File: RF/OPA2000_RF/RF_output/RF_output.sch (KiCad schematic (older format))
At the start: 36 parts, among them J1 Conn_Coaxial, J2 VDD in, J3 GND, Q1 BLF188XR, T1 TLT, T2 TLT, T3 TLT

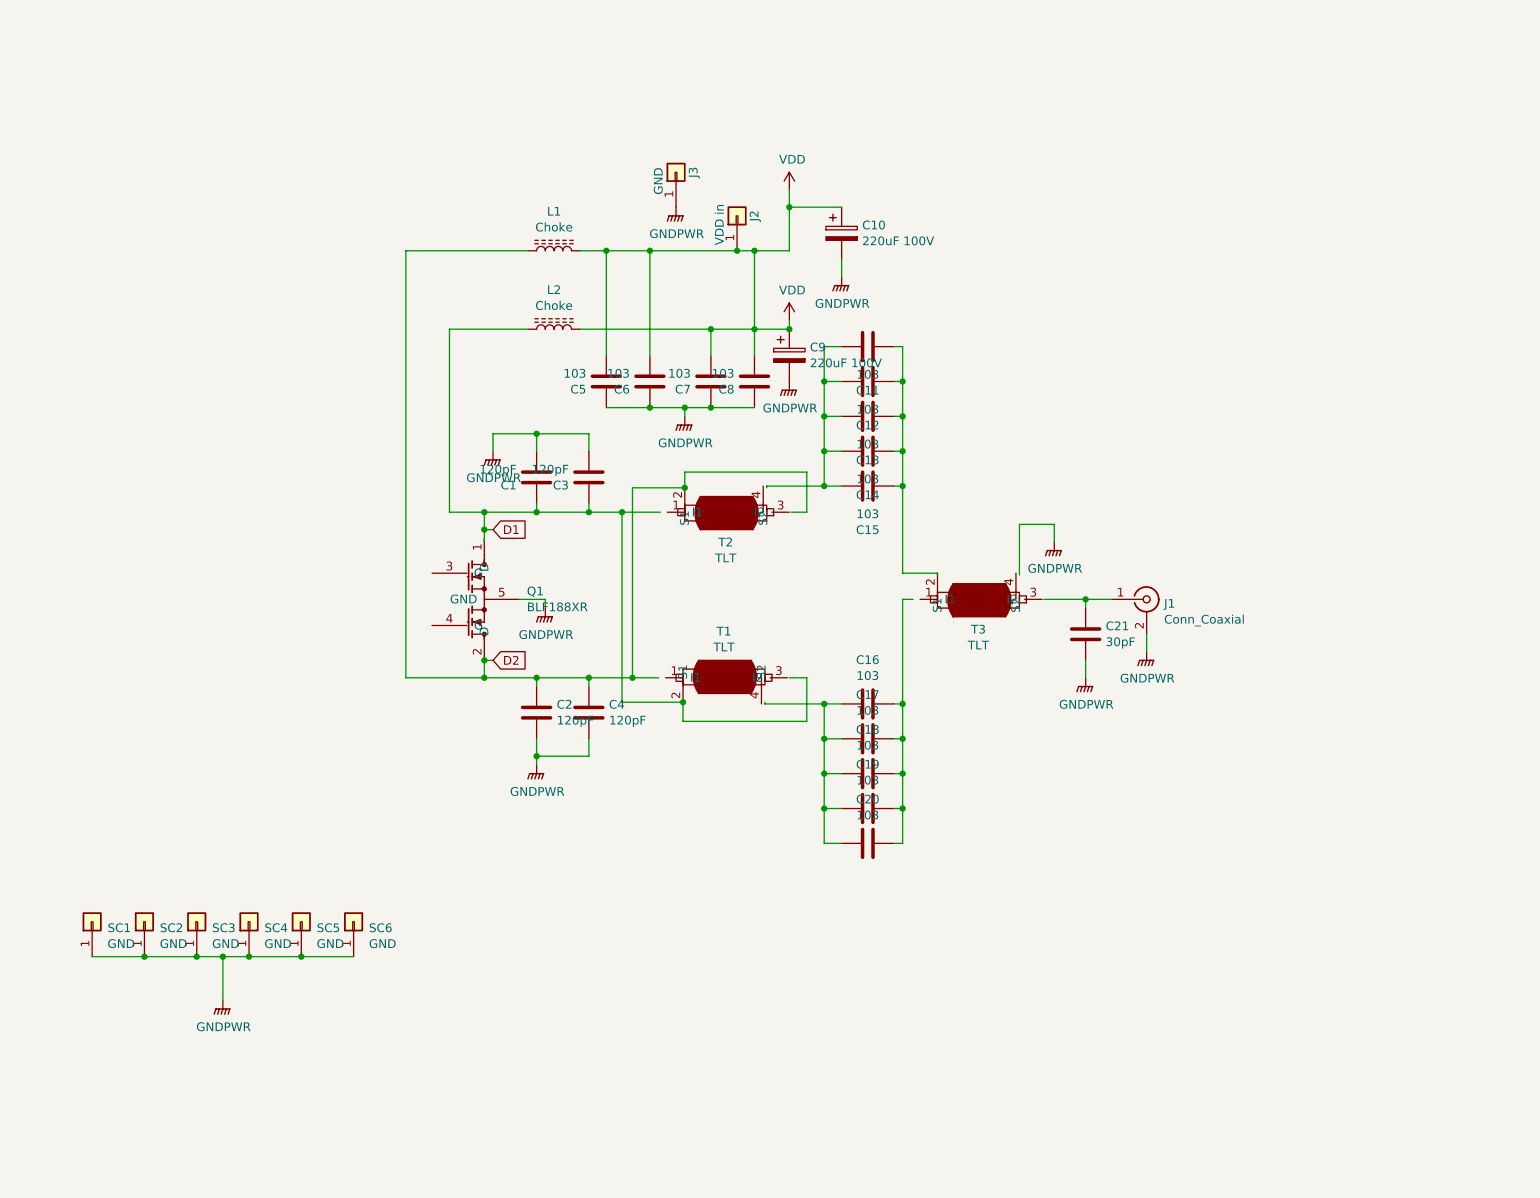
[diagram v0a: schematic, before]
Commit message: MCU2 sch done
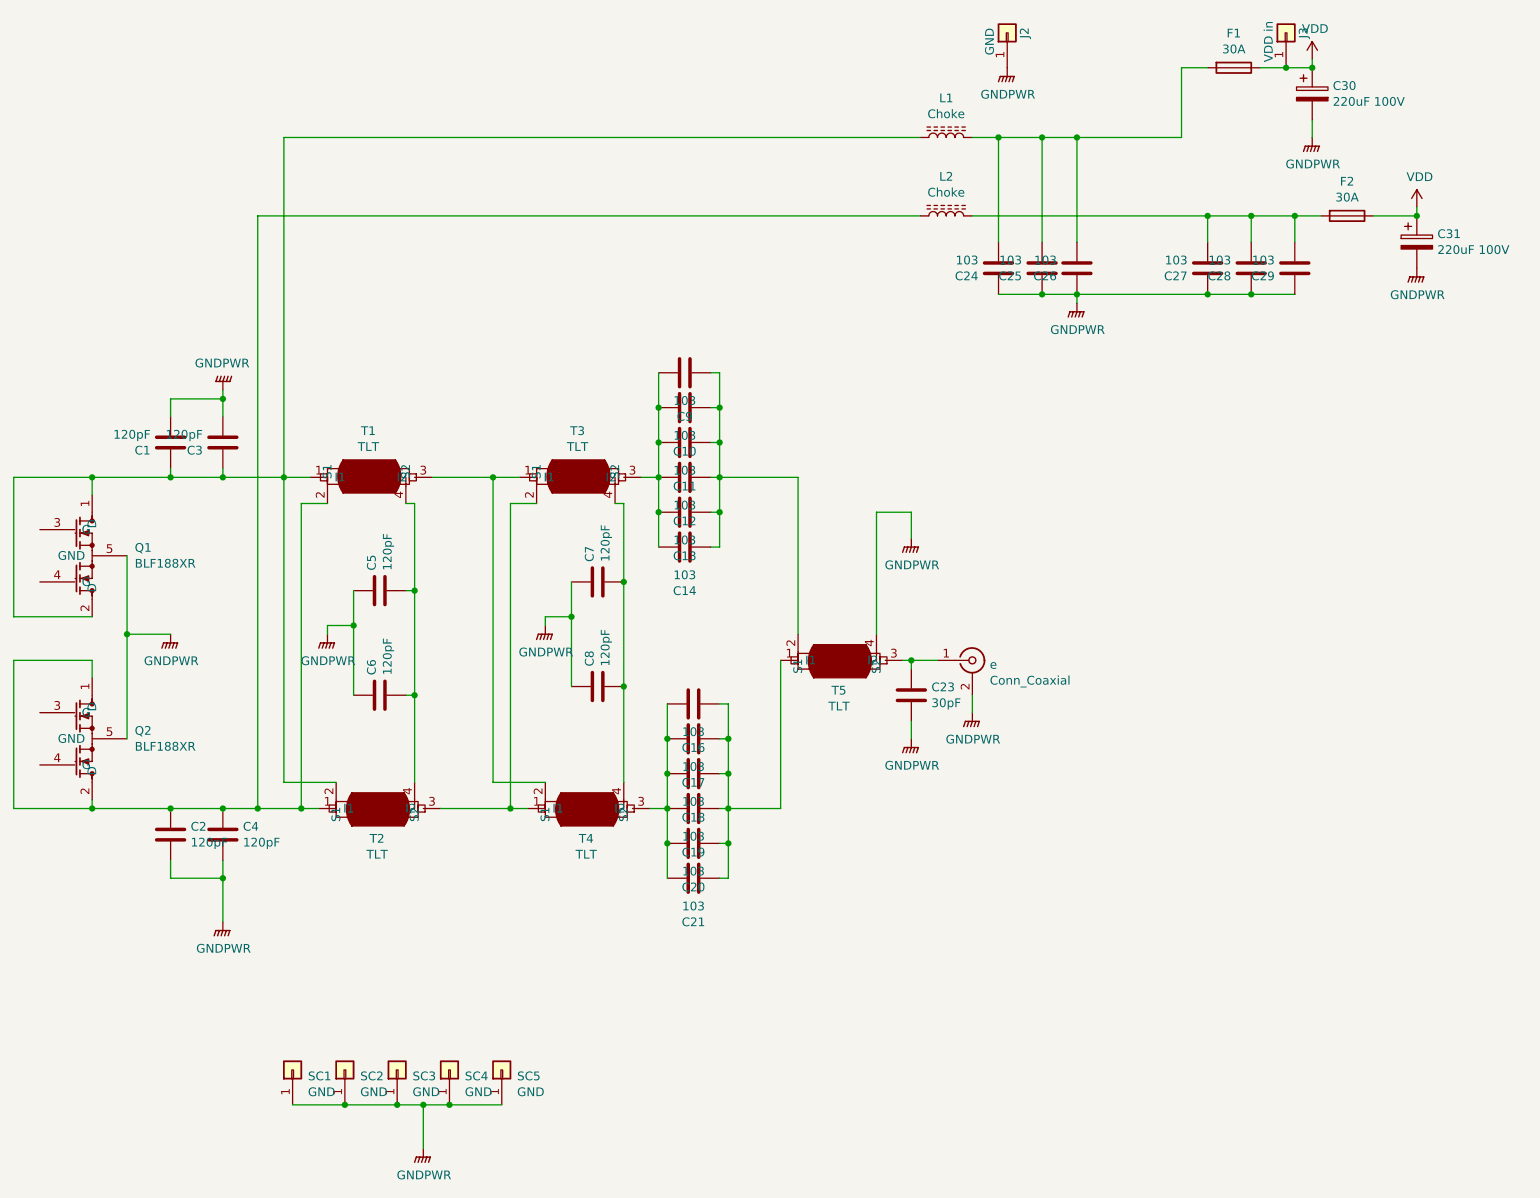
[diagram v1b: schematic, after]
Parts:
- removed C15: 103, Capacitors_SMD:C_1206_HandSoldering, symbol Device:C
- removed SC6: GND, MyPCBLib:M3_Screwhole, symbol Connector_Generic:Conn_01x01
- added C10, C21, C26, C29, C9: 103, Capacitor_SMD:C_1206_3216Metric_Pad1.33x1.80mm_HandSolder, symbol Device:C
- added C5, C6, C7, C8: 120pF, Capacitor_SMD:C_1210_3225Metric_Pad1.33x2.70mm_HandSolder, symbol Device:C
- added F1, F2: 30A, MyPCBLib:Fuseholder_Littelfuse_Nano2_456, symbol Device:Fuse
- added Q2: BLF188XR, MyPCBLib:BLF188XR, symbol MySchLib:BLF188XR
- added T4, T5: TLT, MyPCBLib:Laird_28B1020_100, symbol MyRF:TLT
- C1: renamed from C4; footprint Capacitors_SMD:C_1210_HandSoldering -> Capacitor_SMD:C_1210_3225Metric_Pad1.33x2.70mm_HandSolder
- C11, C12, C13, C14, C16, C17, C18, C19, C20: footprint Capacitors_SMD:C_1206_HandSoldering -> Capacitor_SMD:C_1206_3216Metric_Pad1.33x1.80mm_HandSolder
- C2: renamed from C3; footprint Capacitors_SMD:C_1210_HandSoldering -> Capacitor_SMD:C_1210_3225Metric_Pad1.33x2.70mm_HandSolder
- C23: renamed from C21; footprint Capacitors_SMD:C_1210_HandSoldering -> Capacitor_SMD:C_1210_3225Metric_Pad1.33x2.70mm_HandSolder
- C24: renamed from C5; footprint Capacitors_SMD:C_1206_HandSoldering -> Capacitor_SMD:C_1206_3216Metric_Pad1.33x1.80mm_HandSolder
- C25: renamed from C6; footprint Capacitors_SMD:C_1206_HandSoldering -> Capacitor_SMD:C_1206_3216Metric_Pad1.33x1.80mm_HandSolder
- C27: renamed from C7; footprint Capacitors_SMD:C_1206_HandSoldering -> Capacitor_SMD:C_1206_3216Metric_Pad1.33x1.80mm_HandSolder
- C28: renamed from C8; footprint Capacitors_SMD:C_1206_HandSoldering -> Capacitor_SMD:C_1206_3216Metric_Pad1.33x1.80mm_HandSolder
- C3: renamed from C2; footprint Capacitors_SMD:C_1210_HandSoldering -> Capacitor_SMD:C_1210_3225Metric_Pad1.33x2.70mm_HandSolder
- C30: renamed from C10; footprint Capacitors_SMD:CP_Elec_10x10.5 -> Capacitor_SMD:CP_Elec_10x10.5
- C31: renamed from C9; footprint Capacitors_SMD:CP_Elec_10x10.5 -> Capacitor_SMD:CP_Elec_10x10.5
- C4: renamed from C1; footprint Capacitors_SMD:C_1210_HandSoldering -> Capacitor_SMD:C_1210_3225Metric_Pad1.33x2.70mm_HandSolder
- L1, L2: footprint (none) -> MyPCBLib:5943004901
- T1, T2, T3: footprint (none) -> MyPCBLib:Laird_28B1020_100
- e: renamed from J1; footprint MyPCBLib:RF_conn_pad -> MyPCBLib:RF_conn_pad_short
- renumbered J3 to J2, J2 to J3
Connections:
- net labels removed: D1, D2
- wire segments 130 -> 145
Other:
- moved on the sheet: C1, C2, C23, C24, C25, C27, C28, C3, C30, C31, C4, J2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
